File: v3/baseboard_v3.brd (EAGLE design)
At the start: 100 x 80 mm, 41 parts, among them Q1 18A/40V/5mΩ, U1 MC33926, U2 MC33926, U3 Value

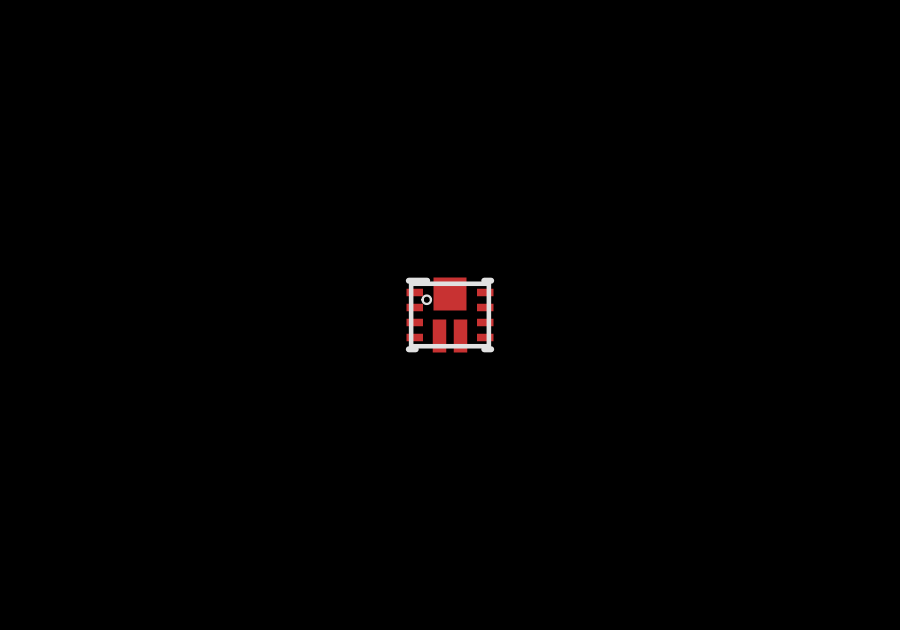
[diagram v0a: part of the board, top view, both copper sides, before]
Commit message: Moving away from bb ideas.
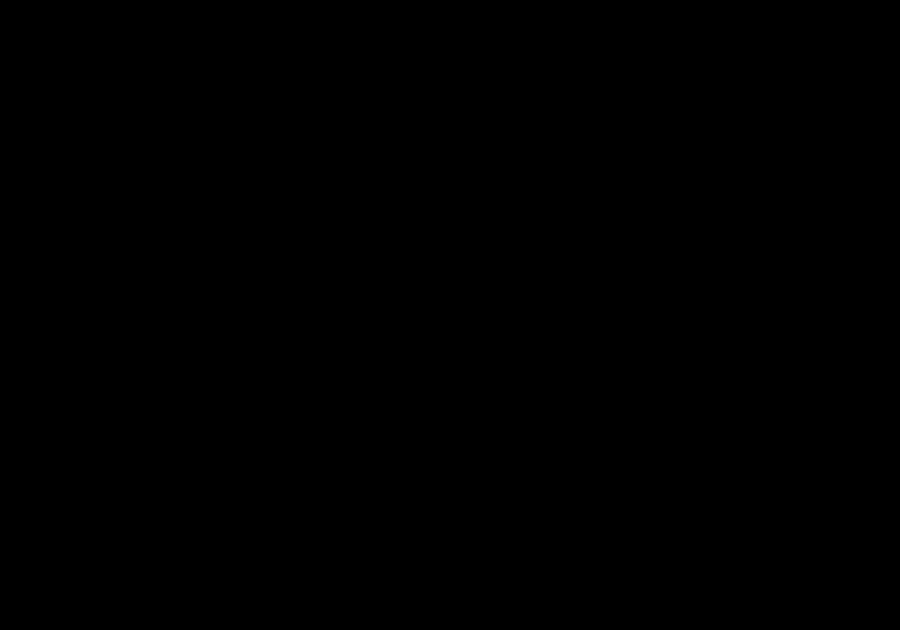
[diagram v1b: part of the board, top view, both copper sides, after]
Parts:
- removed U3: Value, powerbench:RNR0011A
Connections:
- removed net BOOT: U3.10
- removed net GND: U3.5
- removed net SW: U3.11
- removed net VOUT: U3.6
- net VCC: no longer U3.2
- net VIN: no longer U3.9
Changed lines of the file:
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@@
 <?xml version="1.0" encoding="utf-8"?>
 <!DOCTYPE eagle SYSTEM "eagle.dtd">
-<eagle version="8.0.1">
+<eagle version="8.1.0">
 <drawing>
 <settings>
@@
 <attribute name="PROD_ID" value="CAP-00810" x="12.7" y="30.48" size="1.778" layer="27" rot="R180" display="off"/>
 </element>
-<element name="U3" library="powerbench" package="RNR0011A" value="Value" x="55.245" y="40.9575">
-<attribute name="MANUFACTURER_PART_NUMBER" value="TPS61089RNRR" x="55.245" y="40.9575" size="1.778" layer="27" display="off"/>
-<attribute name="PARTNUMBER" value="TPS61089RNRR" x="55.245" y="40.9575" size="1.778" layer="27" display="off"/>
-<attribute name="REFDES" value="RefDes" x="55.245" y="40.9575" size="1.778" layer="27" display="off"/>
-<attribute name="MANUFACTURER_NAME" value="Texas Instruments" x="55.245" y="40.9575" size="1.778" layer="27" display="off"/>
-<attribute name="TYPE" value="TYPE" x="55.245" y="40.9575" size="1.778" layer="27" display="off"/>
-<attribute name="MANUFACTURER" value="Texas Instruments" x="55.245" y="40.9575" size="1.778" layer="27" display="off"/>
-</element>
 </elements>
 <signals>
@@
 <via x="13.97" y="14.9225" extent="1-16" drill="0.3302"/>
 <via x="13.0175" y="14.9225" extent="1-16" drill="0.3302"/>
-<contactref element="U3" pad="9"/>
 <wire x1="19.05" y1="43.307" x2="26.67" y2="43.307" width="0" layer="19" extent="1-1"/>
 <wire x1="19.6725" y1="34.18" x2="19.05" y2="43.307" width="0" layer="19" extent="1-1"/>
@@
 <wire x1="1.27" y1="16.51" x2="13.0175" y2="18.0975" width="0" layer="19" extent="1-1"/>
 <wire x1="32.7025" y1="21.9" x2="19.6725" y2="20.21" width="0" layer="19" extent="1-1"/>
-<wire x1="56.42" y1="41.2075" x2="13.97" y2="7.747" width="0" layer="19" extent="1-1"/>
 </signal>
 <signal name="PGND" airwireshidden="yes">
@@
 <wire x1="8.255" y1="21.59" x2="10.4775" y2="19.3675" width="0.4064" layer="16"/>
 <wire x1="10.4775" y1="19.3675" x2="10.4775" y2="14.82" width="0.4064" layer="16"/>
-<contactref element="U3" pad="2"/>
 <wire x1="8.255" y1="21.59" x2="11.01" y2="34.29" width="0" layer="19" extent="16-16"/>
-<wire x1="54.07" y1="41.2075" x2="10.4775" y2="14.82" width="0" layer="19" extent="1-16"/>
 </signal>
 <signal name="U2NSF">
@@
 <wire x1="1.27" y1="24.13" x2="4.23" y2="24.13" width="0.4064" layer="1"/>
 </signal>
-<signal name="GND">
-<contactref element="U3" pad="5"/>
-</signal>
-<signal name="VOUT">
-<contactref element="U3" pad="6"/>
-</signal>
-<signal name="BOOT">
-<contactref element="U3" pad="10"/>
-</signal>
-<signal name="SW">
-<contactref element="U3" pad="11"/>
-</signal>
 </signals>
